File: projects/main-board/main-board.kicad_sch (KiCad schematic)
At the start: 0 parts

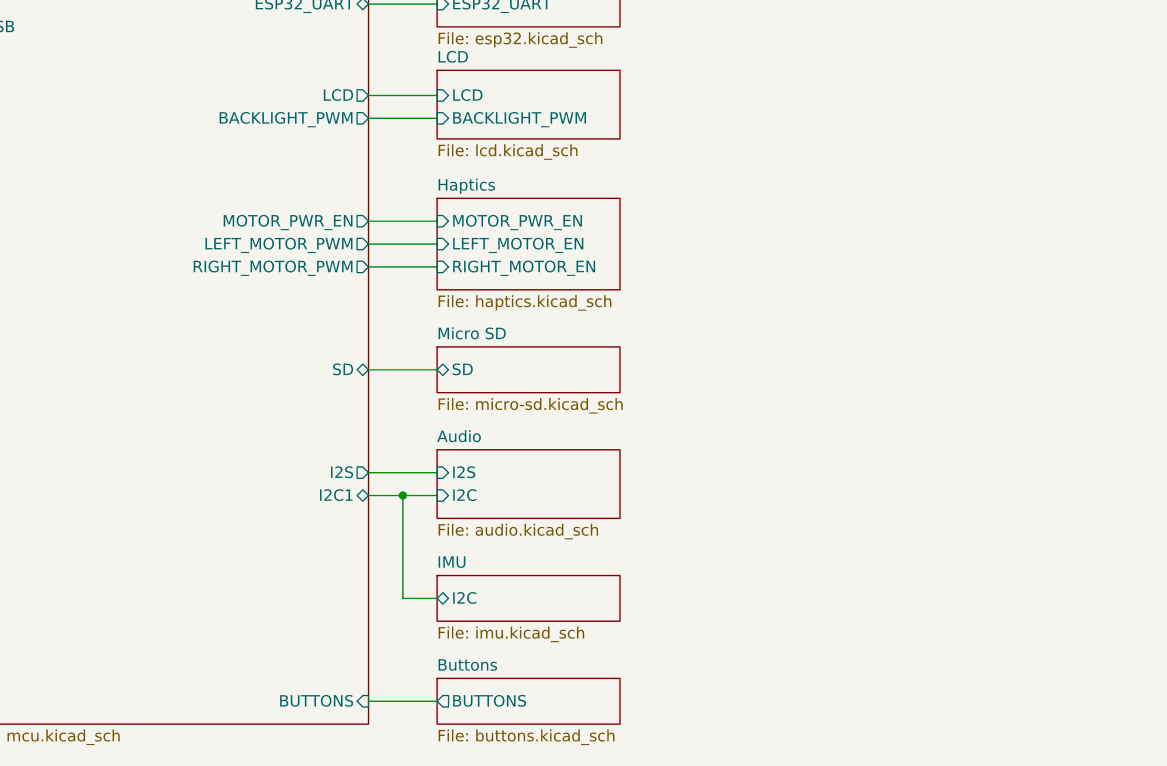
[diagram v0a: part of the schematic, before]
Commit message: WIP splitting main board into 3
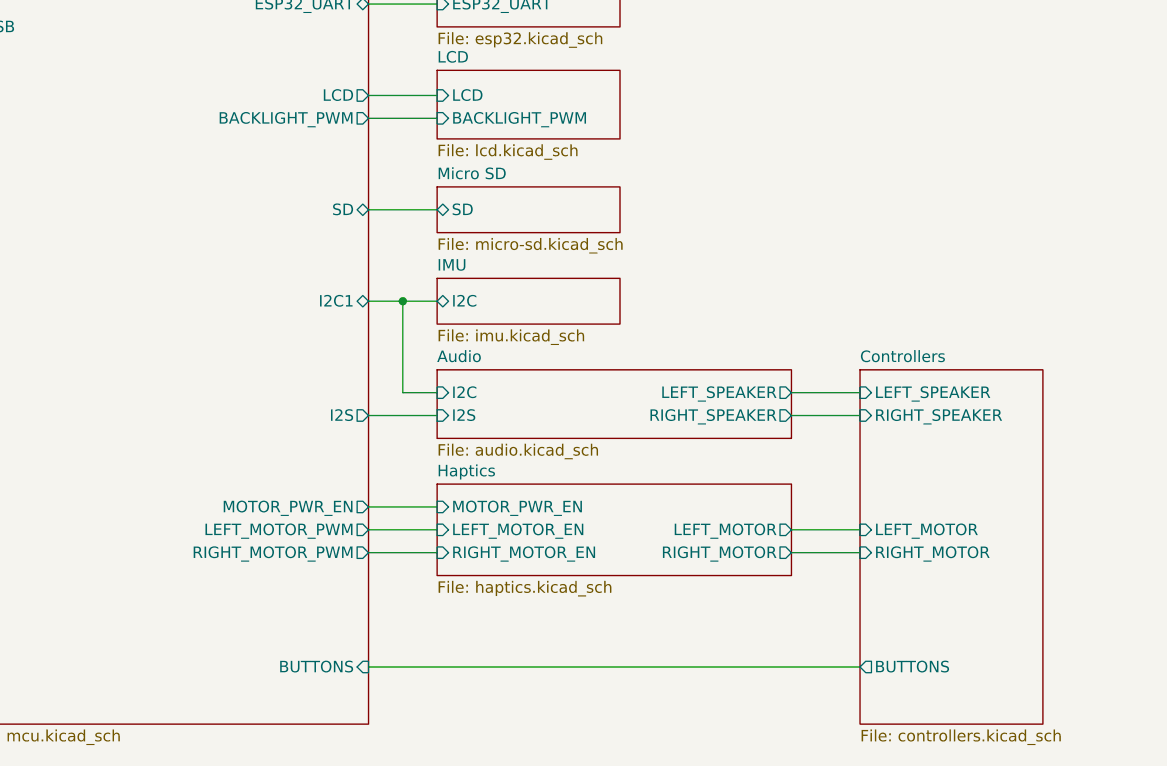
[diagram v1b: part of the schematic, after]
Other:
- removed sheet Buttons
- added sheet Controllers (controllers.kicad_sch)
- sheet Audio ports: added LEFT_SPEAKER, RIGHT_SPEAKER; removed none
- sheet Haptics ports: added LEFT_MOTOR, RIGHT_MOTOR; removed none
